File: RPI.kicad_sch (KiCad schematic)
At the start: 27 parts, among them J1 Conn_01x02_Male, J2 GPIO, J5 Conn_01x06, J6 Conn_01x04, J7 Conn_01x03, J8 Conn_01x02, J9 Conn_01x02, Q1 IRF9540N, Q2 IRF9540N, Q3 BC856BDW1, SW1 SW_SPDT, SW2 SW_SPDT, U1 LM1085-ADJ

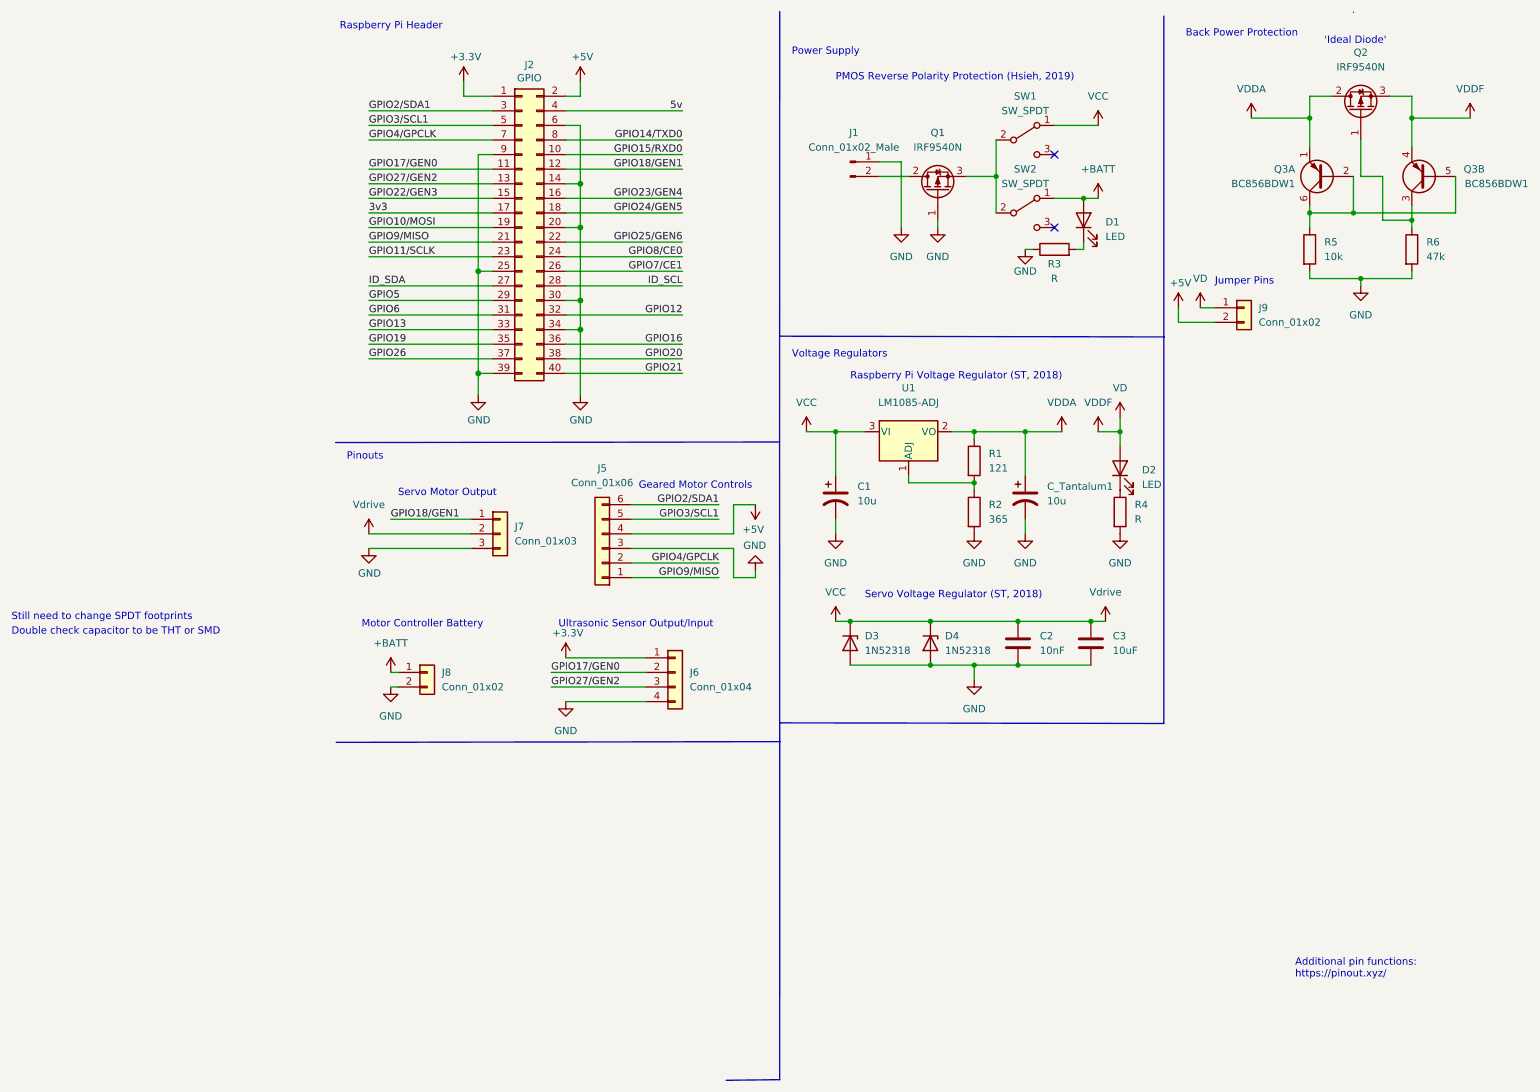
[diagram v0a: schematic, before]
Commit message: Official completion (Maybe add Gerald in)
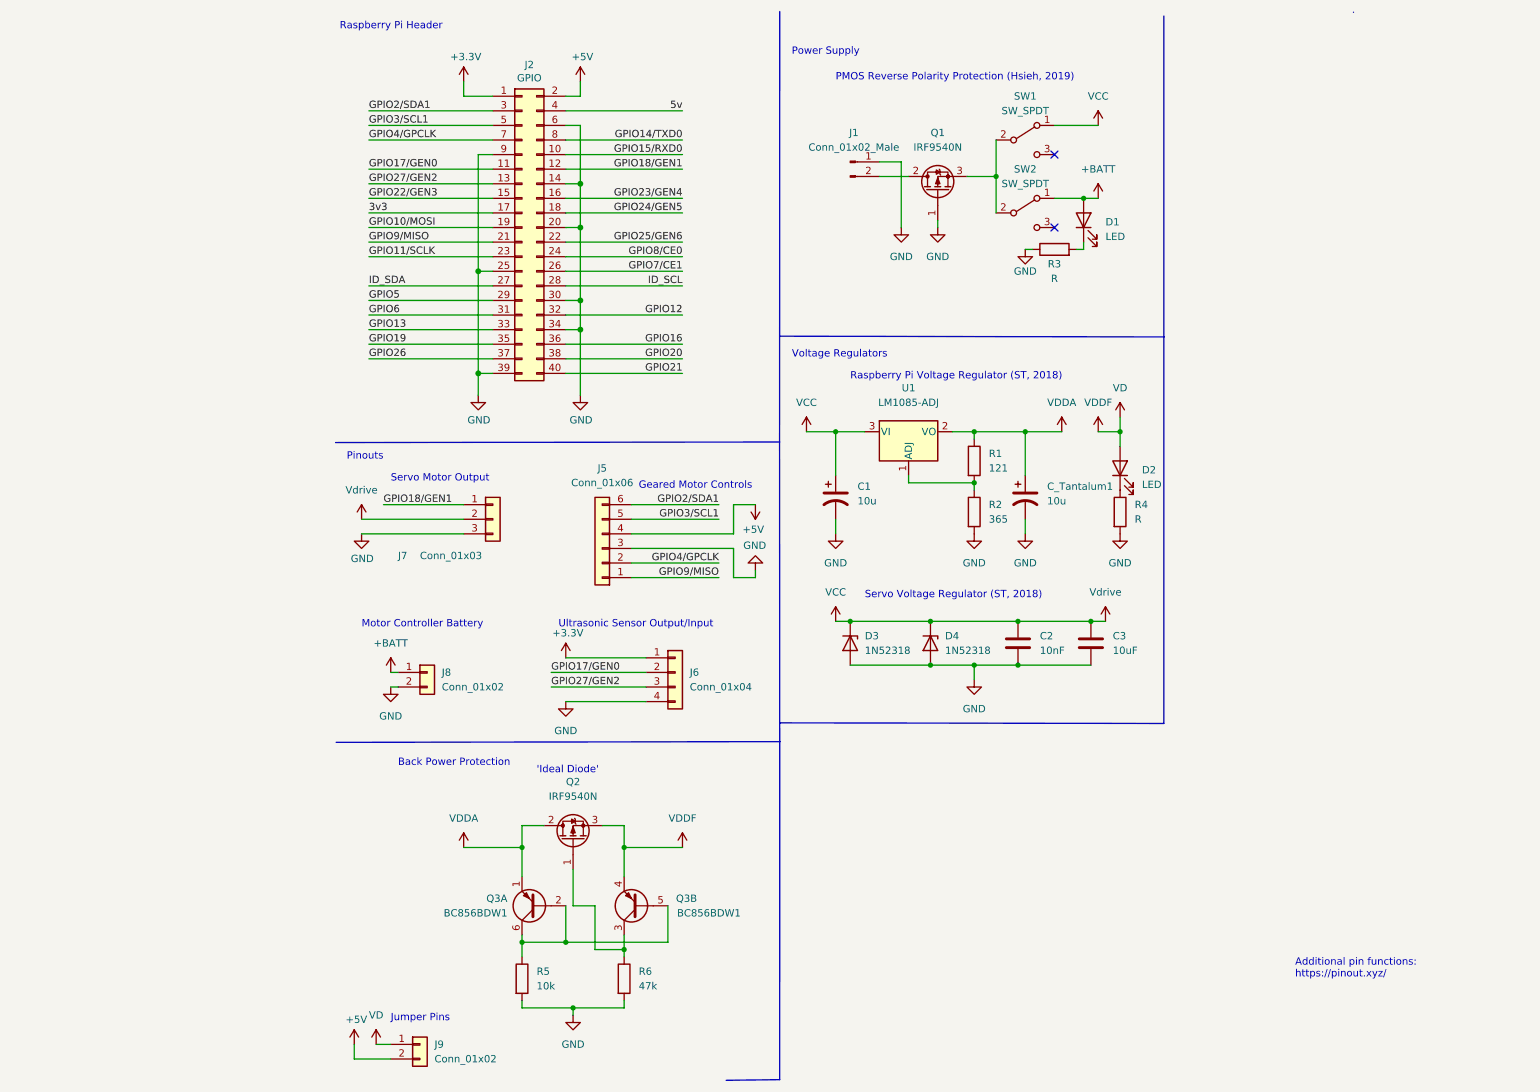
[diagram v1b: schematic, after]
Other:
- note removed: "Double check capacitor to be THT or SMD"
- note removed: "Still need to change SPDT footprints"
- moved on the sheet: J7, J9, Q2, Q3A, Q3B, R5, R6
